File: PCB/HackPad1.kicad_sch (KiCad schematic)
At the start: 25 parts, among them J1 Conn_01x04_Pin, SW1 SW_Push, SW10 RotaryEncoder, SW2 SW_Push, SW3 SW_Push, SW4 SW_Push, SW5 SW_Push, SW6 SW_Push, SW7 SW_Push, SW8 SW_Push, SW9 SW_Push, U1 MOUDLE-SEEEDUINO-XIAO

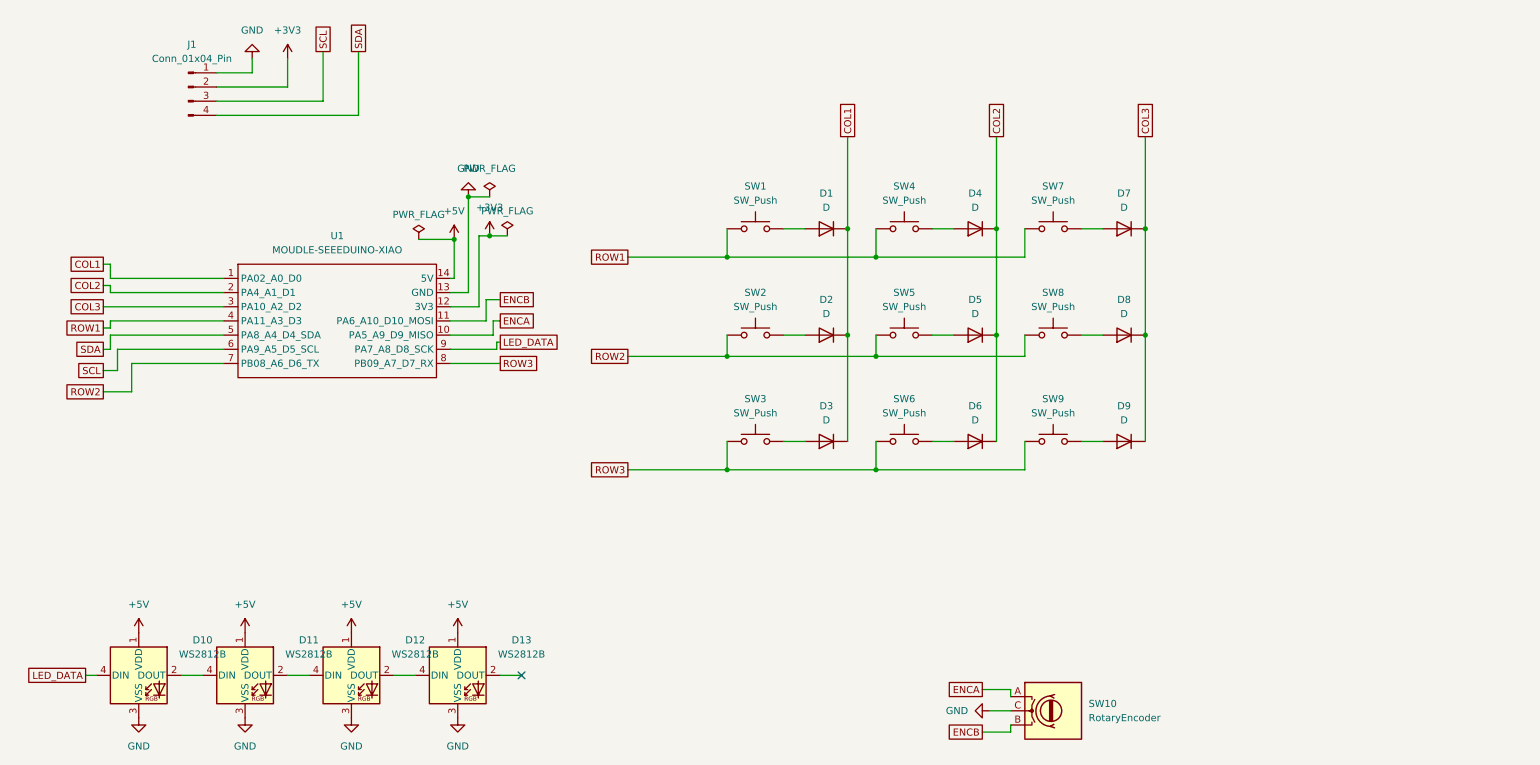
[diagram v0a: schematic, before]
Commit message: Pcb routing
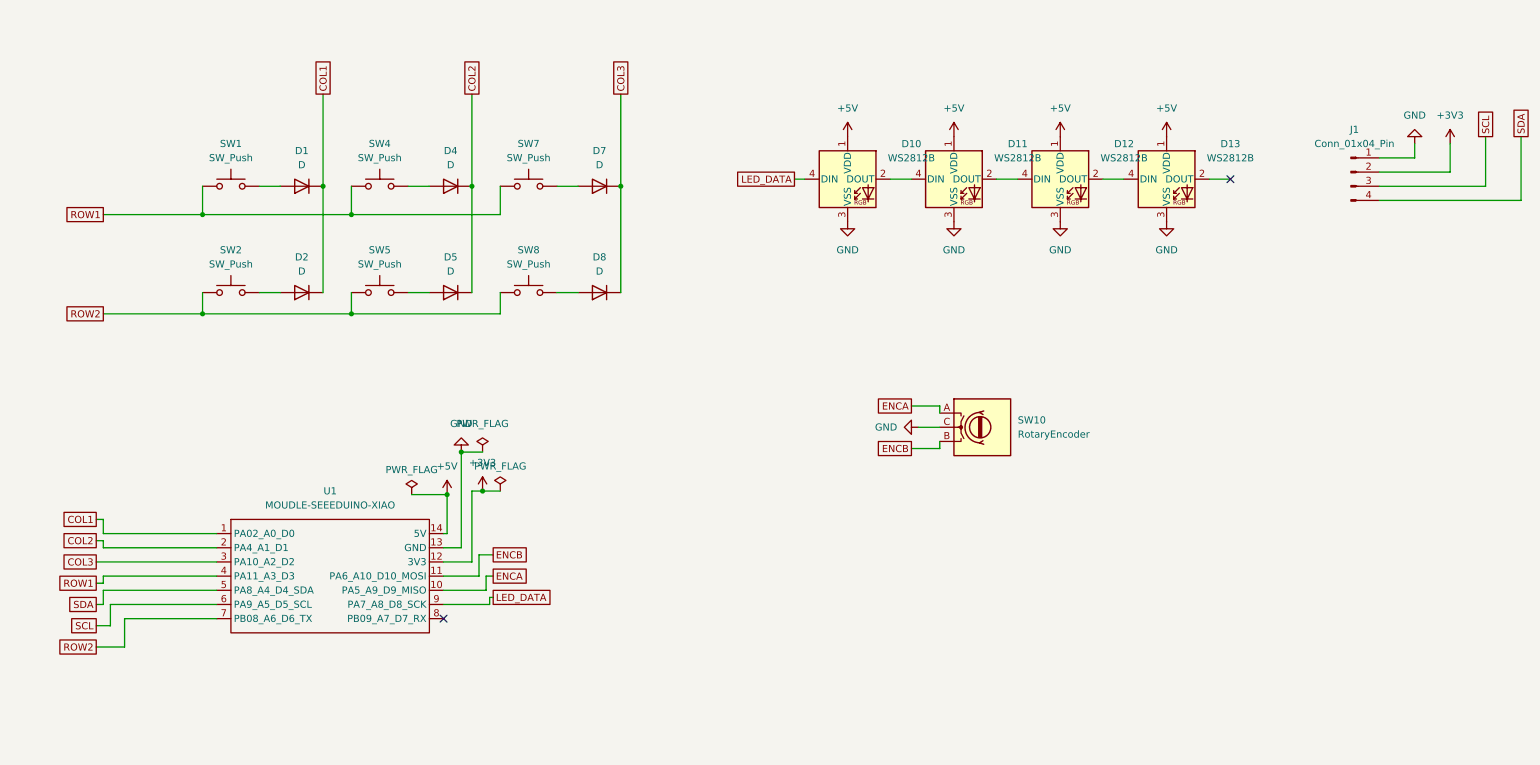
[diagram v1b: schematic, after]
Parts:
- removed D3: D, Diode_THT:D_DO-35_SOD27_P7.62mm_Horizontal, symbol Device:D
- removed D6, D9: D, Diode_THT:D_DO-35_SOD27_P10.16mm_Horizontal, symbol Device:D
- removed SW3, SW6, SW9: SW_Push, Button_Switch_Keyboard:SW_Cherry_MX_1.00u_PCB, symbol Switch:SW_Push
- D10, D11, D12, D13: footprint Keyboard_Parts:MX_SK6812MINI-E -> LED_SMD:LED_SK6812_PLCC4_5.0x5.0mm_P3.2mm
- U1: footprint footprints:XIAO-Generic-Hybrid-14P-2.54-21X17.8MM -> New_XIAO_Series_Footprints:XIAO-SAMD21-DIP
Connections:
- net ROW3: no longer names the net of U1.8 (PB09_A7_D7_RX)
- no-connect marks 1 -> 2
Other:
- moved on the sheet: D1, D10, D11, D12, D13, D2, D4, D5, D7, D8, J1, SW1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
